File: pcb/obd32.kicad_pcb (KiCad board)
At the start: 2 copper layers, 53.8 x 49.3 mm, 71 parts, among them J1 67329-8040, J2 USB_C_Receptacle_USB2.0, J3 OBD2, J4 Conn_02x05_Odd_Even, J5 Conn_02x05_Odd_Even, J6 Micro_SD_Card, J7 U.FL-R-SMT-101, SW1 SW_Push, SW2 SW_Push, SW3 SW_Push, U1 LMR33630BDDA, U2 ESP32-WROOM-32, U3 AZ1117C-3.3, U4 CP2102N-A01-GQFN24, U5 ICM-20689, U6 BMP388, U7 MCP2562-E-MF, U8 SiP32431DR3, U9 MAX-M8W

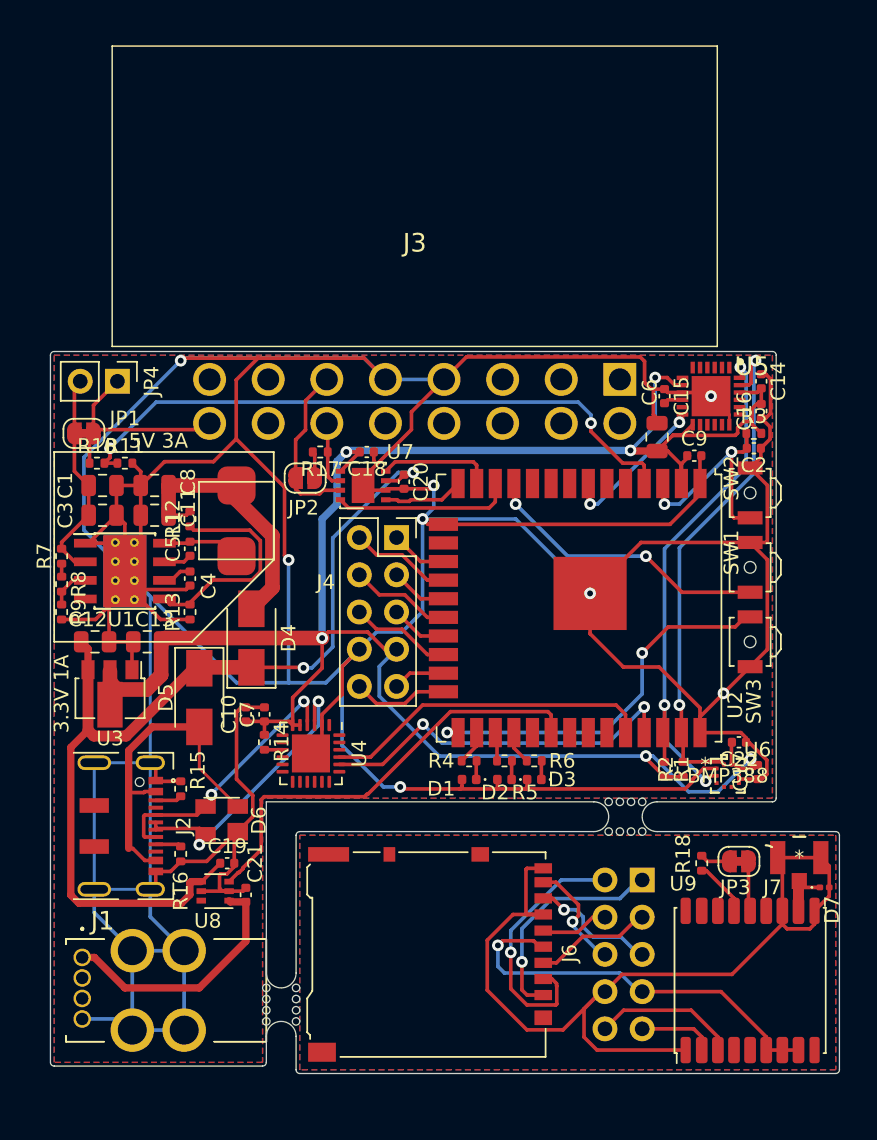
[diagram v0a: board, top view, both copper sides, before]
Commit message: Board: Adjustments
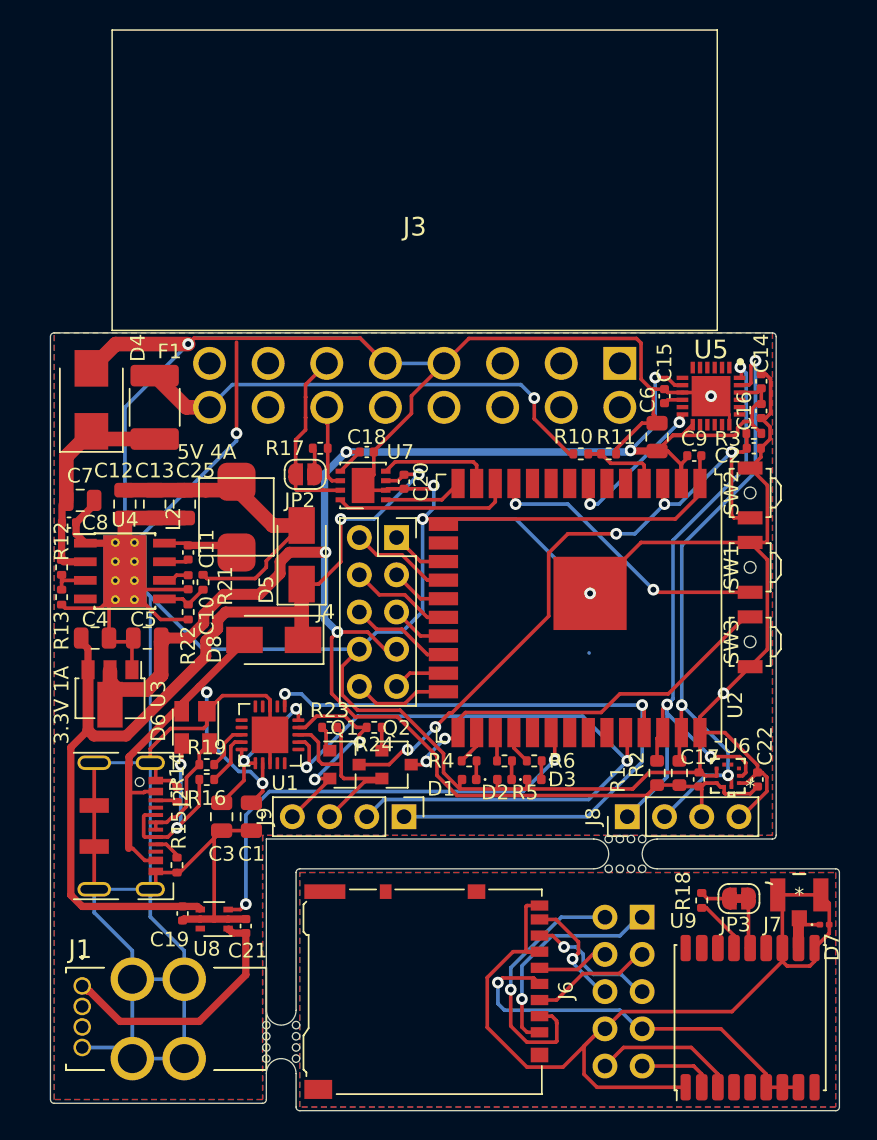
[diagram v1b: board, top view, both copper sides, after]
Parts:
- removed JP1: SolderJumper_2_Bridged, Jumper:SolderJumper-2_P1.3mm_Bridged_RoundedPad1.0x1.5mm
- removed JP4: Jumper_NO_Small, Connector_PinHeader_2.54mm:PinHeader_1x02_P2.54mm_Vertical
- removed L1: 2.2µH, TDK_SPM5030:TDK_SPM5030
- removed R7: 10K, Resistor_SMD:R_0402_1005Metric
- removed R8: 866K, Resistor_SMD:R_0402_1005Metric
- removed R9: 100K, Resistor_SMD:R_0402_1005Metric
- added C25: 22uF, Capacitor_SMD:C_0805_2012Metric, F.Cu at (206.0, 72.6)
- added D8: D_Schottky, Diode_SMD:D_SMA, F.Cu at (212.1, 81.9)
- added F1: Polyfuse, Fuse:Fuse_1812_4532Metric_Castellated, F.Cu at (204.0, 66.0)
- added J8: Conn_01x04_Male, Connector_PinHeader_2.54mm:PinHeader_1x04_P2.54mm_Vertical, F.Cu at (236.2, 94.0)
- added J9: Conn_01x04_Male, Connector_PinHeader_2.54mm:PinHeader_1x04_P2.54mm_Vertical, F.Cu at (221.0, 94.0)
- added L2: 3.3uH 4A 16mR, TDK_SPM5030:TDK_SPM5030, F.Cu at (205.7, 73.7)
- added Q1: BC817, Package_TO_SOT_SMD:SOT-23, F.Cu at (216.9, 90.4)
- added Q2: BC817, Package_TO_SOT_SMD:SOT-23, F.Cu at (220.5, 90.4)
- added R19: 27R, Resistor_SMD:R_0402_1005Metric, F.Cu at (207.5, 90.4)
- added R21: 100K, Resistor_SMD:R_0402_1005Metric, F.Cu at (207.3, 78.0)
- added R22: 24.9K, Resistor_SMD:R_0402_1005Metric, F.Cu at (206.2, 80.0)
- added R23: 10K, Resistor_SMD:R_0402_1005Metric, F.Cu at (215.9, 87.9)
- added R24: 10K, Resistor_SMD:R_0402_1005Metric, F.Cu at (218.9, 87.9)
- added REF**: OSHW-Logo2_9.8x8mm_SilkScreen, Symbol:OSHW-Logo2_9.8x8mm_SilkScreen, B.Cu at (232.4, 82.8)
- C1: value 10µF -> 100nF
- C10: value 0.1µF -> 1uF
- C11: value 22µF -> 0.1uF; footprint Capacitor_SMD:C_0805_2012Metric -> Capacitor_SMD:C_0402_1005Metric
- C12: value 10µF -> 22uF
- C13: value 22µF -> 22uF
- C15: value 0.47µF -> 0.47uF
- C16, C18, C19, C20, C21, C9: value 0.1µF -> 0.1uF
- C2: value 1µF -> 1uF
- C3: value 220nF -> 100nF
- C4: value 1µF -> 10uF; footprint Capacitor_SMD:C_0402_1005Metric -> Capacitor_SMD:C_0805_2012Metric
- C5: value 0.1µF -> 22uF; footprint Capacitor_SMD:C_0402_1005Metric -> Capacitor_SMD:C_0805_2012Metric
- C6: value 10µF -> 10uF
- C7: value 4.7µF -> 10uF 20V; footprint Capacitor_SMD:C_0402_1005Metric -> Capacitor_SMD:C_0805_2012Metric
- C8: value 22µF -> 220nF 20V; footprint Capacitor_SMD:C_0805_2012Metric -> Capacitor_SMD:C_0402_1005Metric
- D4: value D_Schottky -> SM6T18A; footprint Diode_SMD:D_SMA -> Diode_SMD:D_SMB
- R1, R2: footprint Resistor_SMD:R_0402_1005Metric -> Resistor_SMD:R_0603_1608Metric
- R12: value 100K -> 200K
- R13: value 24.9K -> 22K
- R14: value 1K -> 5.1K
- R16: value 5.1K -> 27R
- R4, R5: value 65R -> 64.9R
- R6: value 5R -> 4.99R
- U1: value LMR33630BDDA -> FT231XQ; footprint Package_SO:Texas_HSOP-8-1EP_3.9x4.9mm_P1.27mm_ThermalVias -> Package_DFN_QFN:QFN-20-1EP_4x4mm_P0.5mm_EP2.5x2.5mm
- U4: value CP2102N-A01-GQFN24 -> LMR33640DDDA; footprint Package_DFN_QFN:QFN-24-1EP_4x4mm_P0.5mm_EP2.6x2.6mm -> Package_SO:Texas_HSOP-8-1EP_3.9x4.9mm_P1.27mm_ThermalVias
- U7: value MCP2562-E-MF -> MCP2562FD-E-MF
- moved R10 33.0 mm to (233.0, 69.2)
- moved R11 33.0 mm to (234.9, 69.2)
- moved C1 24.8 mm to (210.6, 94.0), turned to 90 degrees
- moved C3 22.1 mm to (208.5, 94.0), turned to 270 degrees
- moved D4 19.6 mm to (199.6, 65.5)
- moved C7 19.3 mm to (198.9, 72.4), turned to 0 degrees
- moved U4 17.8 mm to (201.9, 77.2), turned to 0 degrees
- moved U1 14.9 mm to (211.8, 88.4), turned to 270 degrees
- moved D5 12.0 mm to (214.0, 76.1), turned to 90 degrees
- moved C10 9.84 mm to (206.2, 78.0), turned to 270 degrees
- moved C12 9.62 mm to (201.9, 72.6), turned to 270 degrees
- moved C13 9.41 mm to (204.0, 72.6), turned to 270 degrees
- moved R12 9.36 mm to (197.6, 77.0)
- moved R13 8.82 mm to (197.6, 79.0), turned to 270 degrees
- moved C4 7.65 mm to (199.9, 81.8), turned to 0 degrees
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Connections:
- C1 pad 1: Net-(C1-Pad1) -> GND
- C1 pad 2: GND -> +5VA
- C10 pad 1: +3V3 -> Net-(C10-Pad1)
- C11 pad 2: GND -> Net-(C11-Pad2)
- C12 pad 1: +5V -> Net-(C12-Pad1)
- C13 pad 1: +3V3 -> Net-(C12-Pad1)
- C3 pad 1: GND -> Net-(C3-Pad1)
- C3 pad 2: Net-(C1-Pad1) -> GND
- C4 pad 1: Net-(C4-Pad1) -> +5V
- C5 pad 1: Net-(C5-Pad1) -> +3V3
- C5 pad 2: Net-(C5-Pad2) -> GND
- C7 pad 1: +3V3 -> Net-(C7-Pad1)
- C8 pad 1: Net-(C11-Pad1) -> Net-(C7-Pad1)
- D4 pad 1: +5V -> Net-(C7-Pad1)
- D4 pad 2: Net-(C11-Pad1) -> GND
- D5 pad 2: +5VA -> Net-(C12-Pad1)
- D6 pad 3: USB_D- -> Net-(D6-Pad3)
- D6 pad 4: USB_D+ -> Net-(D6-Pad4)
- J2 pad A6: USB_D+ -> Net-(D6-Pad4)
- J2 pad A7: USB_D- -> Net-(D6-Pad3)
- J2 pad B6: USB_D+ -> Net-(D6-Pad4)
- J2 pad B7: USB_D- -> Net-(D6-Pad3)
- R12 pad 2: Net-(C11-Pad1) -> Net-(C7-Pad1)
- R13 pad 1: GND -> Net-(R12-Pad1)
- R13 pad 2: Net-(R12-Pad1) -> GND
- R14 pad 1: +3V3 -> GND
- R14 pad 2: Net-(R14-Pad2) -> Net-(J2-PadA5)
- R15 pad 1: GND -> Net-(J2-PadB5)
- R15 pad 2: Net-(J2-PadA5) -> GND
- R16 pad 1: Net-(J2-PadB5) -> Net-(D6-Pad3)
- R16 pad 2: GND -> USB_D-
- U1 pad 1: GND -> UART_TX
- U1 pad 2: Net-(C1-Pad1) -> (no net)
- U1 pad 3: Net-(R8-Pad2) -> GND
- U1 pad 5: Net-(R12-Pad1) -> (no net)
- U1 pad 6: Net-(C4-Pad1) -> (no net)
- U1 pad 7: Net-(C5-Pad1) -> (no net)
- U1 pad 8: Net-(C5-Pad2) -> USB_D+
- U1 pad 9: GND -> USB_D-
- U4 pad 1: (no net) -> GND
- U4 pad 2: GND -> Net-(C7-Pad1)
- U4 pad 3: USB_D+ -> Net-(R12-Pad1)
- U4 pad 4: USB_D- -> (no net)
- U4 pad 5: +3V3 -> Net-(R21-Pad1)
- U4 pad 6: +3V3 -> Net-(C10-Pad1)
- U4 pad 7: (no net) -> Net-(C11-Pad1)
- U4 pad 8: (no net) -> Net-(C11-Pad2)
- U4 pad 9: Net-(R14-Pad2) -> GND
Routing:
- net ADC: track 43.7 -> 5.39 mm, vias 2 -> 0
- net ESP32_EN: track 15.6 -> 46.6 mm, vias 2 -> 5
- net UART_RX: track 22.0 -> 48.3 mm, vias 0 -> 2
- net UART_TX: track 24.7 -> 49.3 mm
- net Net-(C12-Pad1): track 0.00 -> 21.7 mm
- net +BATT: track 14.6 -> 32.9 mm, vias 0 -> 1
- net USB_D+: track 19.9 -> 3.16 mm, vias 2 -> 0
- net Net-(C11-Pad1): track 18.3 -> 1.68 mm
- net Net-(C7-Pad1): track 0.00 -> 15.8 mm
- net /USB-to-Serial/DTR: track 0.00 -> 15.4 mm
- net /USB-to-Serial/RTS: track 0.00 -> 15.2 mm, vias 0 -> 2
- net Net-(C1-Pad1): track 14.7 -> 0.00 mm
- net Net-(D6-Pad3): track 0.00 -> 14.6 mm, vias 0 -> 2
- net USB_D-: track 17.6 -> 3.59 mm, vias 2 -> 0
- net Net-(R12-Pad1): track 15.0 -> 2.68 mm
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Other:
- board size 53.8 x 49.3 mm -> 53.8 x 53.1 mm
- board text added: "5V 4A"
- board text added: "OBD32"
- board text added: "by Malte Schröder"
- board text removed: "5V 3A"
